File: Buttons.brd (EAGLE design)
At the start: 85 x 79 mm, 63 parts, among them T1 SI2301, U1 TCA8418RTWR, U2 Tiny85-20-SMT

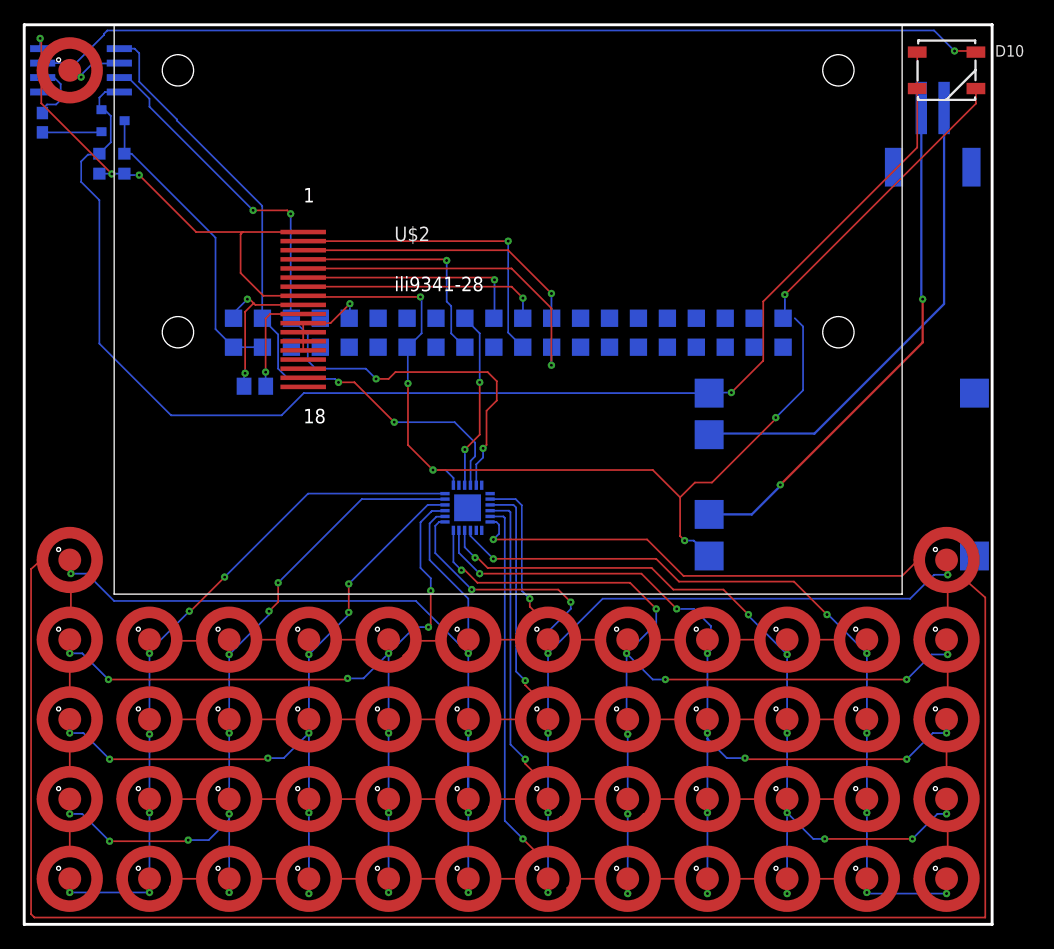
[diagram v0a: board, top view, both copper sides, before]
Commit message: this could be the one neo!
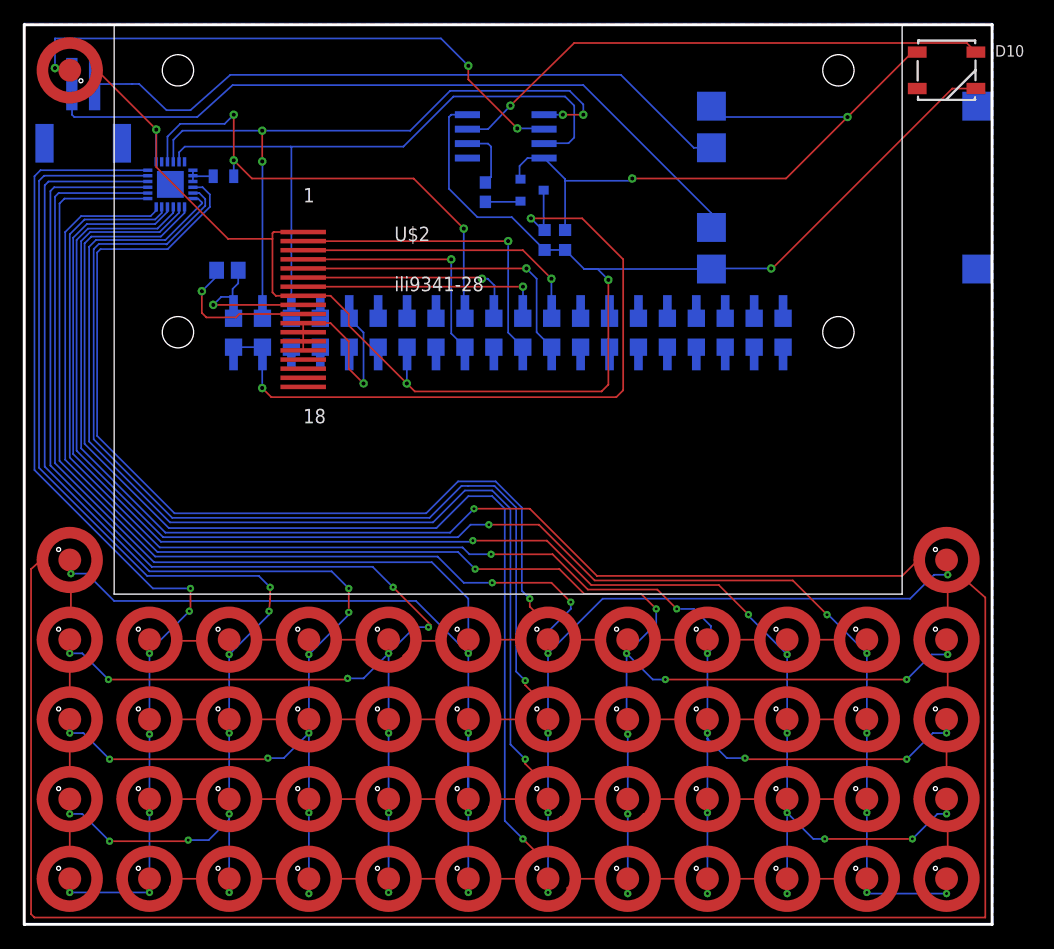
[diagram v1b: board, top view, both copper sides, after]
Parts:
- added R3: 1k, SparkFun-Passives:0805
- R1: value 100 -> 1k
- moved CN1 74.6 mm to (5.18, 70.1)
- moved C11 41.4 mm to (47.5, 60.1)
- moved R2 39.4 mm to (40.5, 64.3)
- moved U1 38.6 mm to (12.8, 65.0)
- moved U2 37.7 mm to (42.3, 69.2)
- moved C10 37.5 mm to (45.7, 60.1)
- moved T1 37.3 mm to (44.6, 64.5)
- moved U$1 25.2 mm to (59.0, 56.2)
- moved R1 10.5 mm to (17.8, 57.4), turned to 180 degrees
- turned U$3 to 180 degrees
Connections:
- removed net N$49: U1.8
- removed net N$9: U1.7
- new net N$8: R3.2, U1.1, U1.2, U1.3
- net 3V3@2: now also R3.1
- net N$24: now also U1.4; no longer U1.2
- net N$29: now also U1.5; no longer U1.3
- net N$30: now also U1.6; no longer U1.4
- net N$31: now also U1.7; no longer U1.5
- net N$33: now also U1.8; no longer U1.6
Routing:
- net N$9: track 0.00 -> 164.1 mm
- net N$30: track 118.3 -> 188.1 mm
- net N$29: track 111.9 -> 181.5 mm
- net N$24: track 106.2 -> 175.7 mm
- net N$31: track 125.3 -> 194.3 mm
- net N$33: track 275.9 -> 343.1 mm
- net N$23: track 73.7 -> 140.3 mm
- net N$46: track 76.9 -> 141.9 mm
- net N$45: track 79.2 -> 143.8 mm
- net N$44: track 85.0 -> 149.1 mm
- net N$43: track 87.5 -> 151.0 mm
- net N$42: track 87.4 -> 150.7 mm
- net N$11: track 122.0 -> 59.0 mm, vias 1 -> 2
- net N$41: track 73.7 -> 133.6 mm
- net N$40: track 69.1 -> 122.4 mm
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- added copper zone on layer 16, net N$13
- added copper zone on layer 1, net N$14
